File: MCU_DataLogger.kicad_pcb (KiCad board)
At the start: 2 copper layers, 50.8 x 30.5 mm, 30 parts, among them J1 Conn_01x04_Pin, J2 Conn_01x04_Pin, J3 Conn_01x09_Pin, J4 Conn_02x03_Odd_Even, U1 24LC1025, U2 24LC1025, U3 ATMEGA328P-AU, U4 DS1337S_, Y1 32.768 KHz, Y2 16 MHz

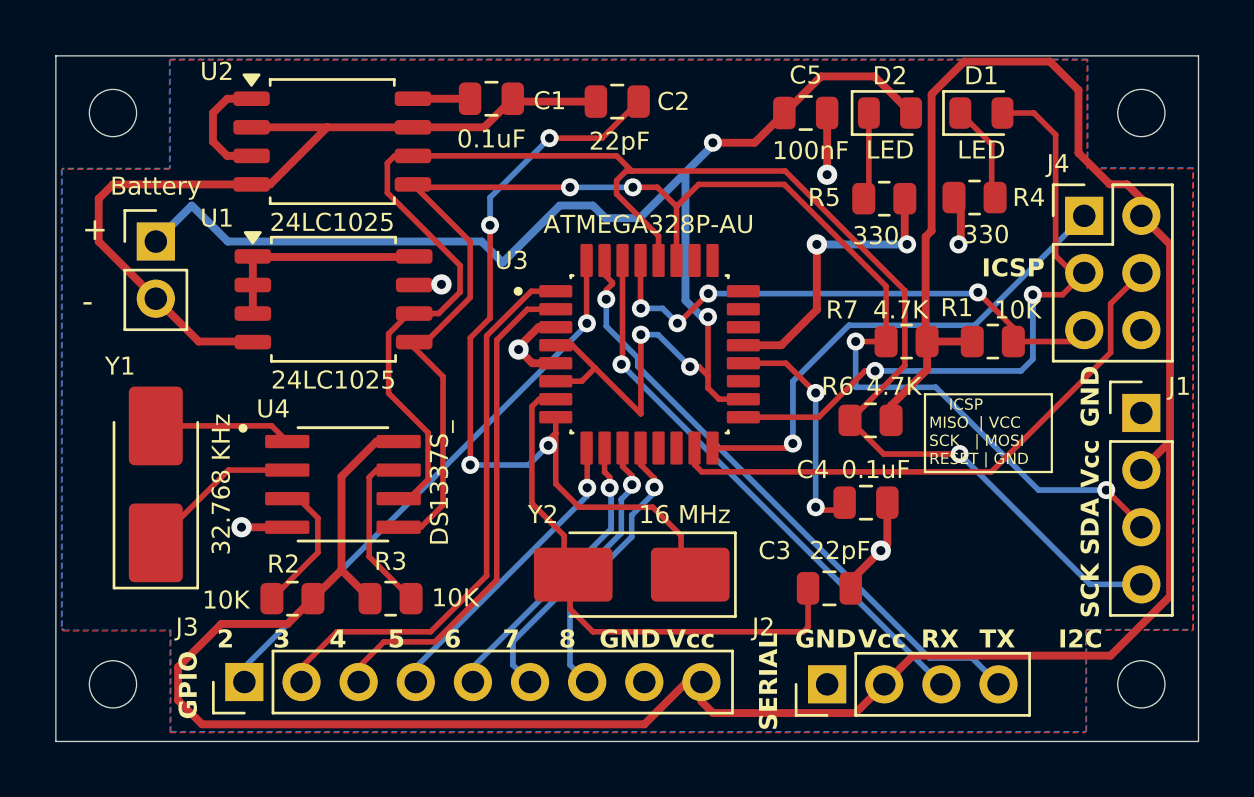
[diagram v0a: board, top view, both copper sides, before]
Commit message: 4-layer PCB complete
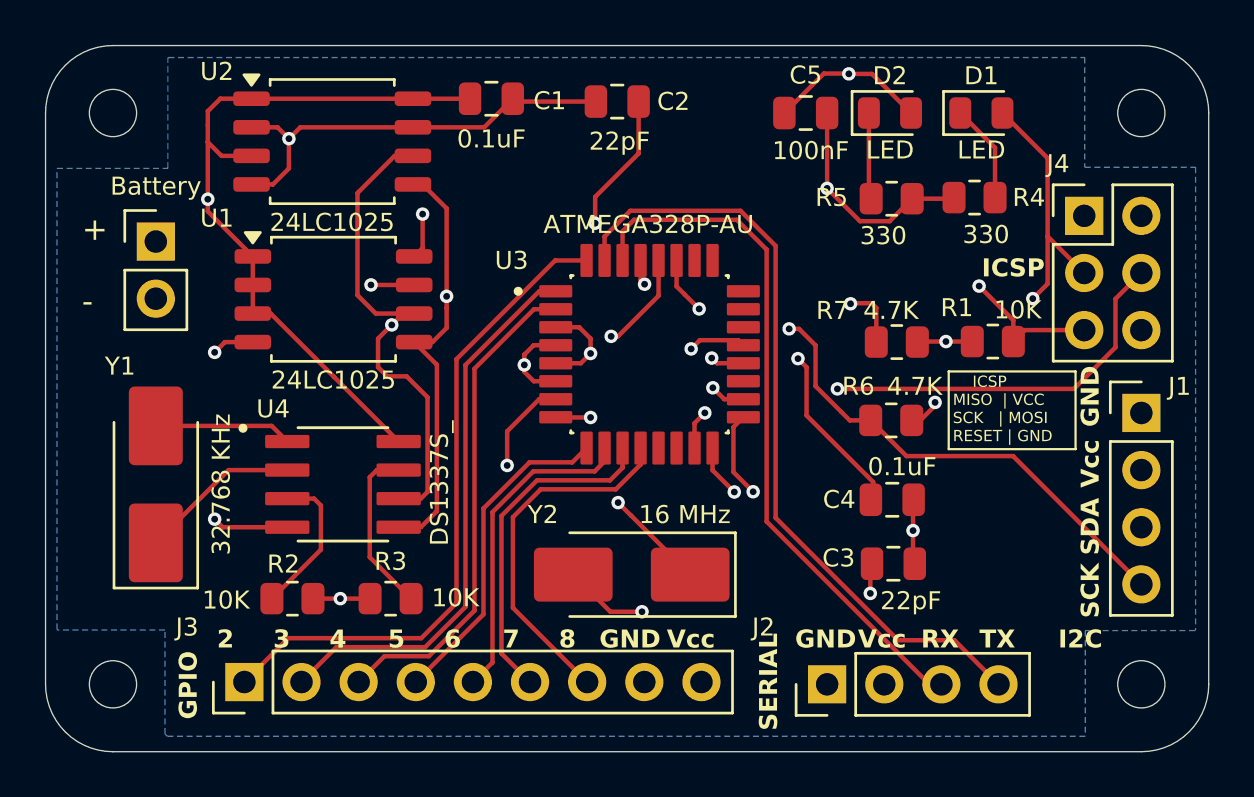
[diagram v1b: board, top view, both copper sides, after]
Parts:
- moved C3 3.05 mm to (106.1, 101.5)
- moved C4 1.17 mm to (106.1, 98.7)
- moved R6 0.92 mm to (106.0, 95.2)
- moved R7 0.44 mm to (106.3, 91.7)
- moved R5 0.33 mm to (106.0, 85.3)
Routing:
- net VCC: track 203.3 -> 53.8 mm, vias 4 -> 8
- net GND: track 67.8 -> 46.4 mm
- net Net-(U3-PB7): track 36.5 -> 26.5 mm, vias 4 -> 3
- net /SCL: track 74.8 -> 66.1 mm, vias 1 -> 3
- net /TX: track 27.4 -> 34.9 mm, vias 1 -> 0
- net /RX: track 24.8 -> 31.3 mm, vias 1 -> 0
- net Net-(U3-PB6): track 23.8 -> 29.2 mm, vias 0 -> 3
- net /SDA: track 66.8 -> 62.1 mm, vias 4 -> 3
- net /D2: track 25.1 -> 29.3 mm, vias 1 -> 0
- net /D8: track 12.5 -> 16.1 mm, vias 1 -> 0
- net Net-(U3-AREF): track 10.3 -> 13.5 mm
- net /SCK: track 29.2 -> 32.2 mm
- net /D7: track 13.1 -> 15.1 mm, vias 1 -> 0
- net /RESET: track 24.2 -> 22.5 mm, vias 4 -> 2
- net /D6: track 13.1 -> 14.4 mm, vias 1 -> 0
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- added copper zone on In2.Cu, net VCC
- removed copper zone on F.Cu, net VCC
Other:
- board size 50.8 x 30.5 mm -> 51.7 x 31.4 mm
- copper layers 2 -> 4
